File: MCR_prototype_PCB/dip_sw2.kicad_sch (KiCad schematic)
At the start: 10 parts, among them SW2 SW_DIP_x08, U7 74AHC165

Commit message: Add files via upload
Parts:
- R84, R85, R86, R87, R88, R89, R90, R91: footprint (none) -> Resistor_SMD:R_0805_2012Metric; KiLib_Generator (none) -> SMD_2terminal_chip_molded
- SW2: footprint (none) -> Button_Switch_THT:SW_DIP_SPSTx08_Slide_9.78x22.5mm_W7.62mm_P2.54mm; KiLib_Generator (none) -> button_switch/DIP
- U7: footprint (none) -> Package_SO:SOIC-16_3.9x9.9mm_P1.27mm; KiLib_Generator (none) -> package/gullwing
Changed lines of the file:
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@@
 			)
 		)
-		(property "Footprint" ""
+		(property "Footprint" "Button_Switch_THT:SW_DIP_SPSTx08_Slide_9.78x22.5mm_W7.62mm_P2.54mm"
 			(at 55.88 71.12 0)
 			(hide yes)
@@
 			)
 		)
+		(property "KiLib_Generator" "button_switch/DIP"
+			(at 55.88 71.12 0)
+			(hide yes)
+			(show_name no)
+			(do_not_autoplace no)
+			(effects
+				(font
+					(size 1.27 1.27)
+				)
+			)
+		)
 		(pin "12"
 		)
@@
 			)
 		)
-		(property "Footprint" ""
+		(property "Footprint" "Resistor_SMD:R_0805_2012Metric"
 			(at 80.01 52.07 0)
 			(hide yes)
@@
 			)
 		)
+		(property "KiLib_Generator" "SMD_2terminal_chip_molded"
+			(at 80.01 52.07 0)
+			(hide yes)
+			(show_name no)
+			(do_not_autoplace no)
+			(effects
+				(font
+					(size 1.27 1.27)
+				)
+			)
+		)
 		(pin "1"
 		)
@@
 			)
 		)
-		(property "Footprint" ""
+		(property "Footprint" "Resistor_SMD:R_0805_2012Metric"
 			(at 92.71 52.07 0)
 			(hide yes)
@@
 			)
 		)
+		(property "KiLib_Generator" "SMD_2terminal_chip_molded"
+			(at 92.71 52.07 0)
+			(hide yes)
+			(show_name no)
+			(do_not_autoplace no)
+			(effects
+				(font
+					(size 1.27 1.27)
+				)
+			)
+		)
 		(pin "1"
 		)
@@
 			)
 		)
-		(property "Footprint" ""
+		(property "Footprint" "Resistor_SMD:R_0805_2012Metric"
 			(at 67.31 52.07 0)
 			(hide yes)
@@
 		)
 		(property "Description" "Resistor, small US symbol"
+			(at 67.31 52.07 0)
+			(hide yes)
+			(show_name no)
+			(do_not_autoplace no)
+			(effects
+				(font
+					(size 1.27 1.27)
+				)
+			)
+		)
+		(property "KiLib_Generator" "SMD_2terminal_chip_molded"
 			(at 67.31 52.07 0)
 			(hide yes)
@@
 			)
 		)
-		(property "Footprint" ""
+		(property "Footprint" "Resistor_SMD:R_0805_2012Metric"
 			(at 111.76 52.07 0)
 			(hide yes)
@@
 			)
 		)
+		(property "KiLib_Generator" "SMD_2terminal_chip_molded"
+			(at 111.76 52.07 0)
+			(hide yes)
+			(show_name no)
+			(do_not_autoplace no)
+			(effects
+				(font
+					(size 1.27 1.27)
+				)
+			)
+		)
 		(pin "1"
 		)
@@
 			)
 		)
-		(property "Footprint" ""
+		(property "Footprint" "Resistor_SMD:R_0805_2012Metric"
 			(at 99.06 52.07 0)
 			(hide yes)
@@
 			)
 		)
+		(property "KiLib_Generator" "SMD_2terminal_chip_molded"
+			(at 99.06 52.07 0)
+			(hide yes)
+			(show_name no)
+			(do_not_autoplace no)
+			(effects
+				(font
+					(size 1.27 1.27)
+				)
+			)
+		)
 		(pin "1"
 		)
@@
 			)
 		)
-		(property "Footprint" ""
+		(property "Footprint" "Resistor_SMD:R_0805_2012Metric"
 			(at 86.36 52.07 0)
 			(hide yes)
@@
 		)
 		(property "Description" "Resistor, small US symbol"
+			(at 86.36 52.07 0)
+			(hide yes)
+			(show_name no)
+			(do_not_autoplace no)
+			(effects
+				(font
+					(size 1.27 1.27)
+				)
+			)
+		)
+		(property "KiLib_Generator" "SMD_2terminal_chip_molded"
 			(at 86.36 52.07 0)
 			(hide yes)
@@
 			)
 		)
-		(property "Footprint" ""
+		(property "Footprint" "Package_SO:SOIC-16_3.9x9.9mm_P1.27mm"
 			(at 177.8 115.57 0)
 			(hide yes)
@@
 		)
 		(property "Description" "Shift Register, 8-bit, Parallel Load"
+			(at 177.8 115.57 0)
+			(hide yes)
+			(show_name no)
+			(do_not_autoplace no)
+			(effects
+				(font
+					(size 1.27 1.27)
+				)
+			)
+		)
+		(property "KiLib_Generator" "package/gullwing"
 			(at 177.8 115.57 0)
 			(hide yes)
@@
 			)
 		)
-		(property "Footprint" ""
+		(property "Footprint" "Resistor_SMD:R_0805_2012Metric"
 			(at 105.41 52.07 0)
 			(hide yes)
@@
 		)
 		(property "Description" "Resistor, small US symbol"
+			(at 105.41 52.07 0)
+			(hide yes)
+			(show_name no)
+			(do_not_autoplace no)
+			(effects
+				(font
+					(size 1.27 1.27)
+				)
+			)
+		)
+		(property "KiLib_Generator" "SMD_2terminal_chip_molded"
 			(at 105.41 52.07 0)
 			(hide yes)
@@
 			)
 		)
-		(property "Footprint" ""
+		(property "Footprint" "Resistor_SMD:R_0805_2012Metric"
 			(at 73.66 52.07 0)
 			(hide yes)
@@
 			(at 73.66 52.07 0)
 			(hide yes)
+			(show_name no)
+			(do_not_autoplace no)
+			(effects
+				(font
+					(size 1.27 1.27)
+				)
+			)
+		)
+		(property "KiLib_Generator" "SMD_2terminal_chip_molded"
+			(at 73.66 52.07 0)
+			(hide yes)

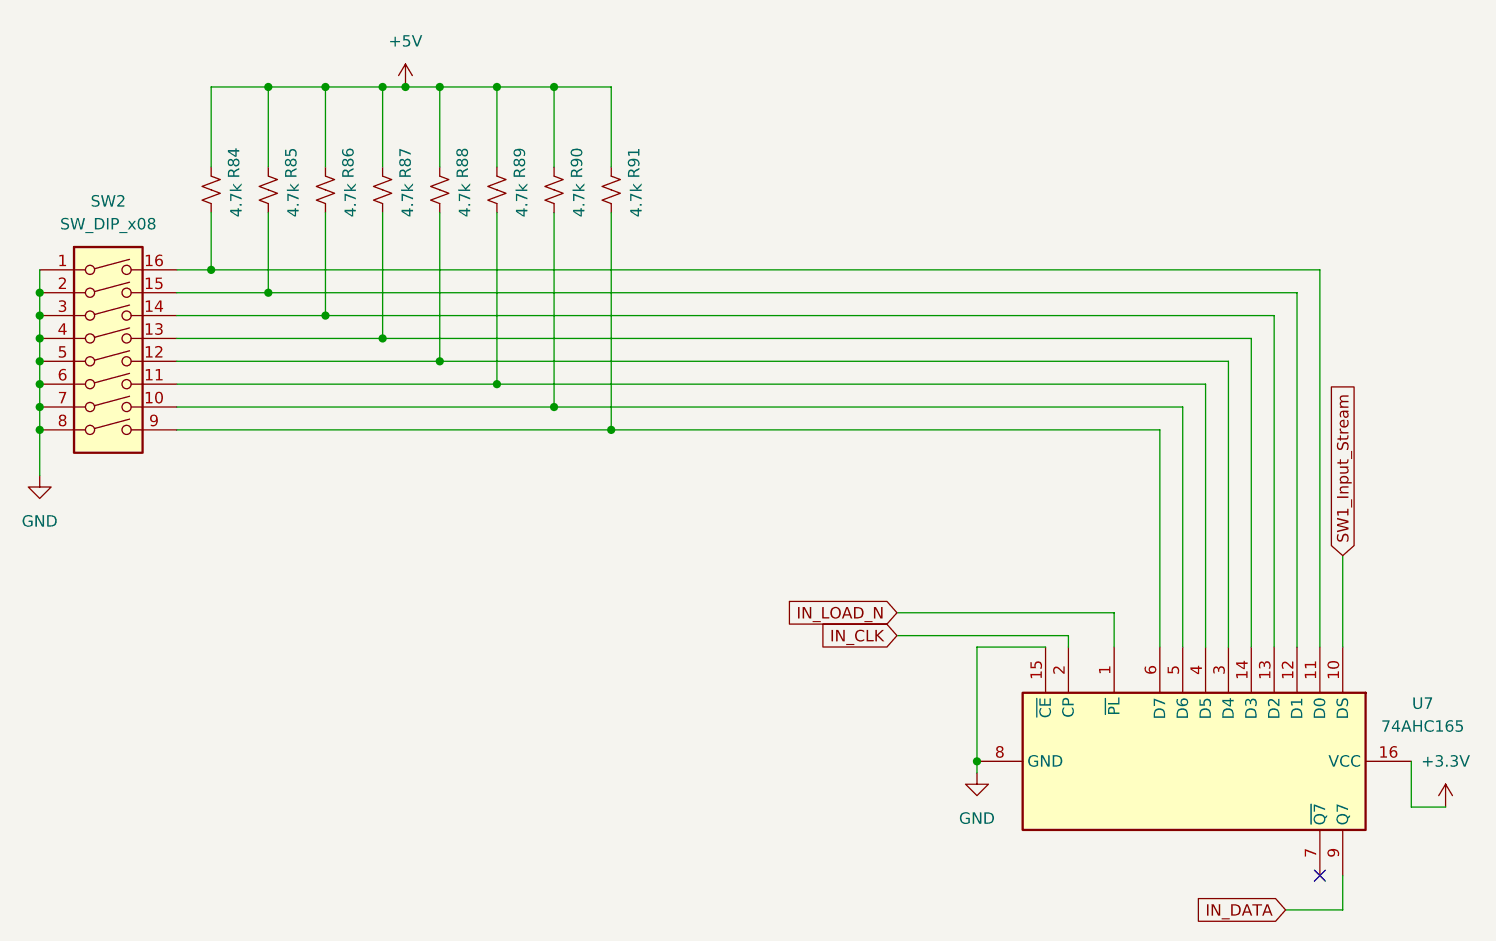
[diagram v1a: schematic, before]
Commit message: Updated 8/22/26
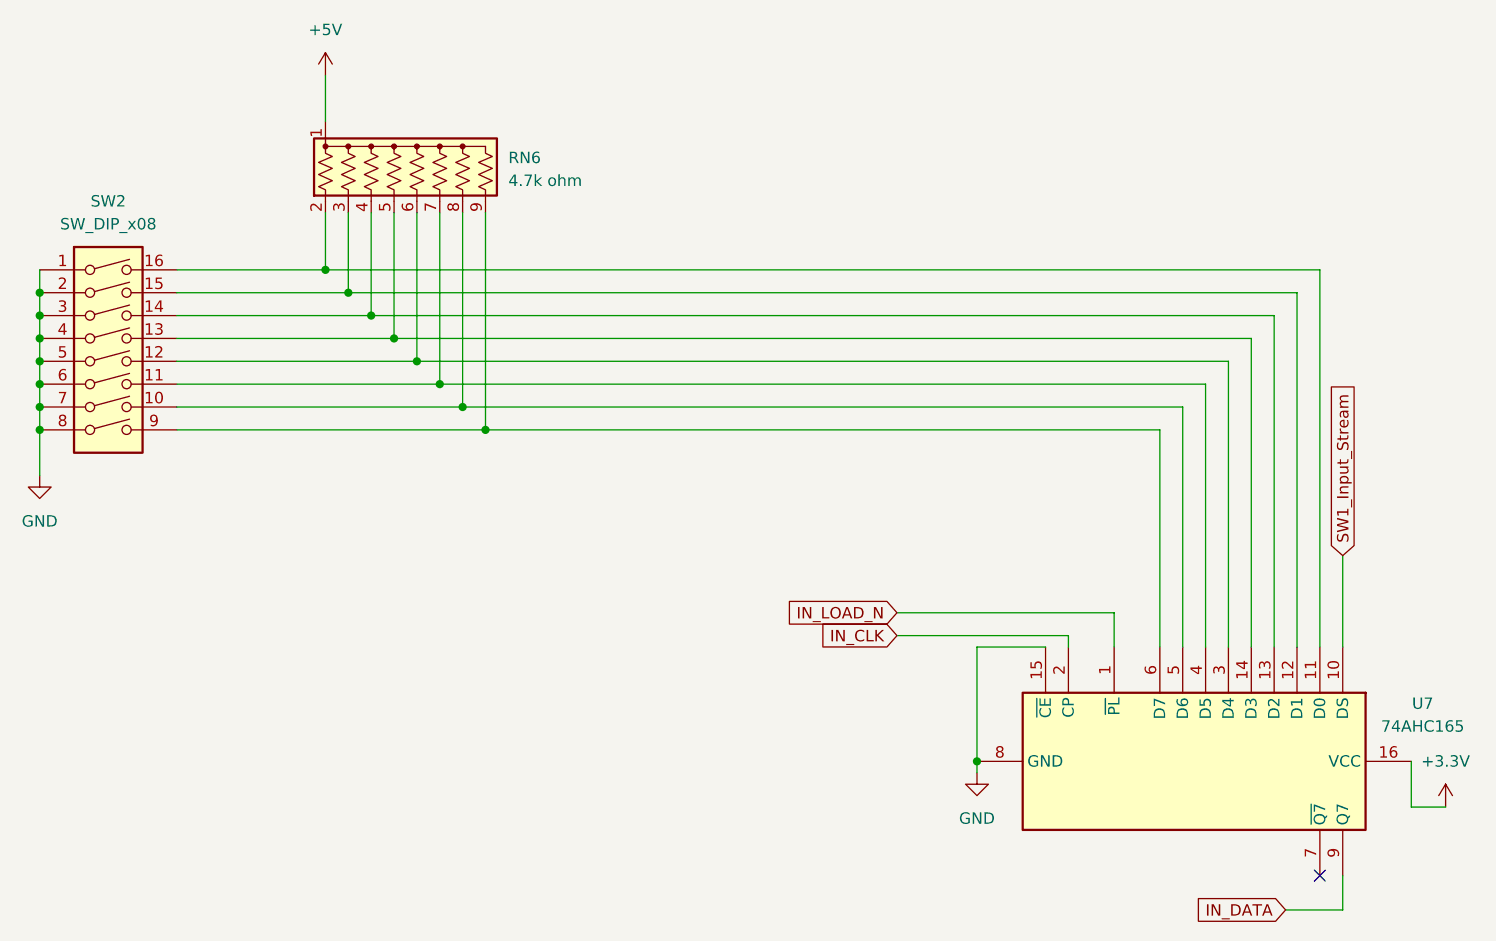
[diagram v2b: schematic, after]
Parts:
- removed R84, R85, R86, R87, R88, R89, R90, R91: 4.7k, Resistor_SMD:R_0805_2012Metric, symbol Device:R_Small_US
- added RN6: 4.7k ohm, Resistor_THT:R_Array_SIP9, symbol Device:R_Network08_US
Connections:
- net +5V: now also RN6.1 (common)
- net at SW2.10, U7.5 (D6): now also RN6.8 (R7)
- net at SW2.11, U7.4 (D5): now also RN6.7 (R6)
- net at SW2.12, U7.3 (D4): now also RN6.6 (R5)
- net at SW2.13, U7.14 (D3): now also RN6.5 (R4)
- net at SW2.14, U7.13 (D2): now also RN6.4 (R3)
- net at SW2.15, U7.12 (D1): now also RN6.3 (R2)
- net at SW2.16, U7.11 (D0): now also RN6.2 (R1)
- net at SW2.9, U7.6 (D7): now also RN6.9 (R8)
